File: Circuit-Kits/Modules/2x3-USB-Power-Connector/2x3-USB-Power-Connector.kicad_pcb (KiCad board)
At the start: 2 copper layers, 23.6 x 15.6 mm, 5 parts, among them J1 MICRO-B, U1 MIC5365 3.3V

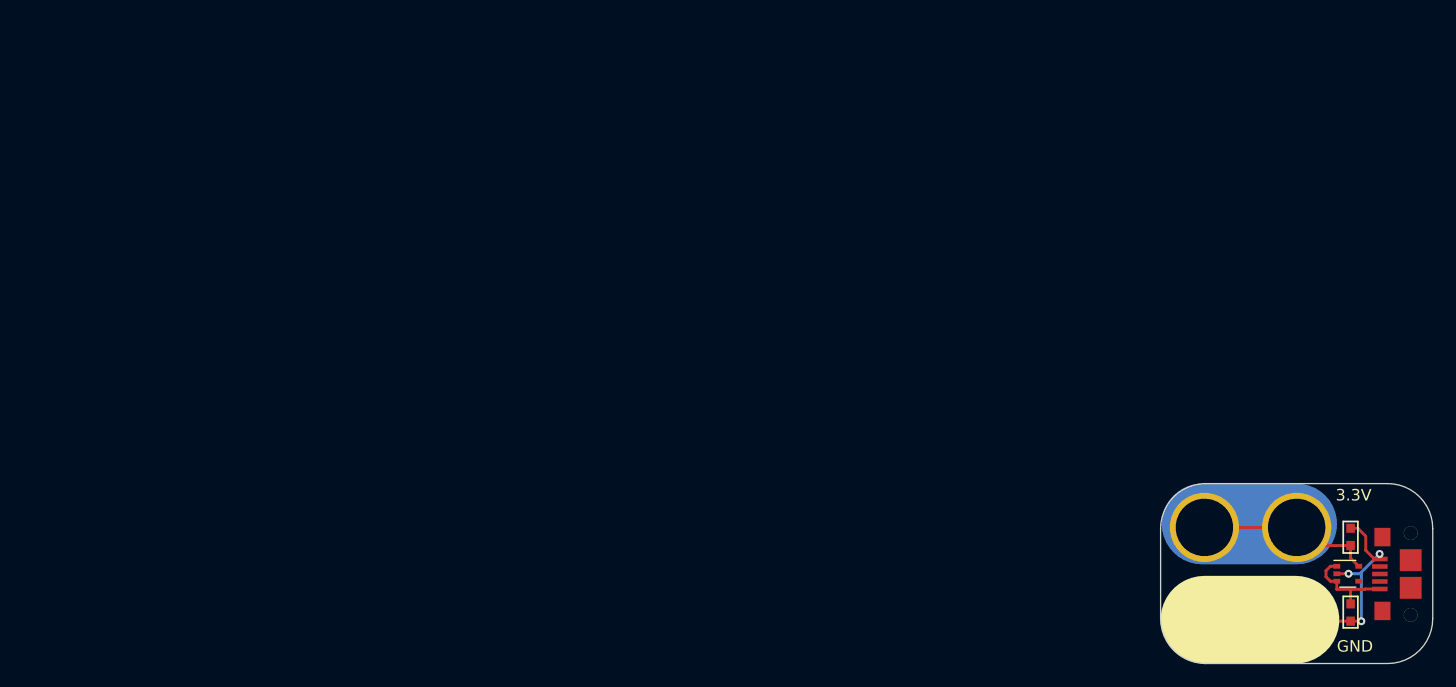
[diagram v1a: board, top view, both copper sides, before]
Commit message: Public release.
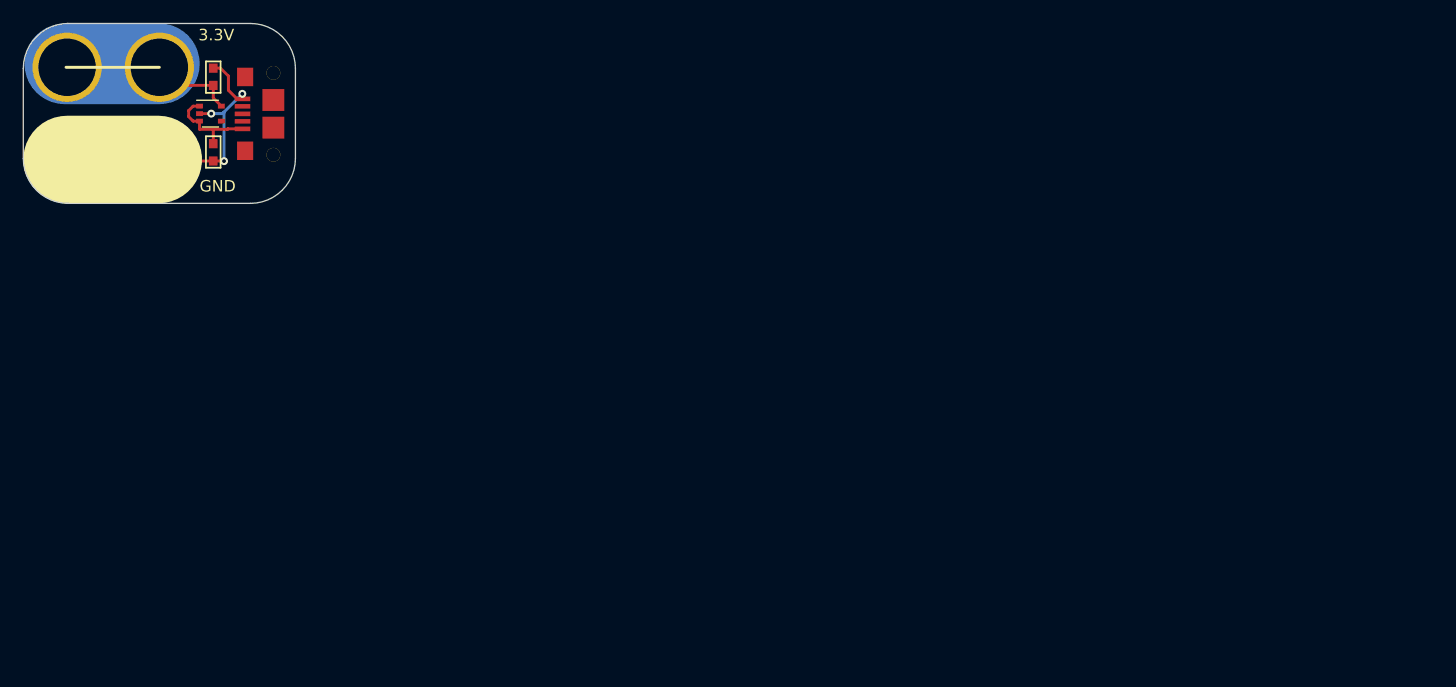
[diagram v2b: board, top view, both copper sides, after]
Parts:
- moved J1 106.4 mm to (42.8, 57.1)
- moved C1 106.4 mm to (37.5, 60.5)
- moved C2 106.4 mm to (37.5, 53.9)
- moved U1 106.4 mm to (37.3, 57.1)
- moved J1 106.4 mm to (32.9, 61.1)
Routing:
- net (no net): track 16.0 -> 8.00 mm
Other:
- board text added: "FABRICATION NOTES 1. THIS IS A 2 LAYER BOARD. 2. EXTERNAL LAYERS SHALL HAVE 1 OZ COPPER. 3. MATERIAL: FR4 AND 0.062 INCH +/- 10% THICK. 4. BOARDS SHALL BE ROHS COMPLIANT. 5. MANUFACTURE IN ACCORDANCE WITH IPC-6012 CLASS 2 6. MASK: BOTH SIDES OF THE BOARD SHALL HAVE SOLDER MASK (ORANGE) OVER BARE COPPER. 7. SILK: BOTH SIDES OF THE BOARD SHALL HAVE WHITE SILK. DO NOT PLACE SILK OVER BARE COPPER. 8.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"
